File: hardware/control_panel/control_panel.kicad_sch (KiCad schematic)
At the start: 6 parts, among them SW1 RotaryEncoder_Switch_MP, SW2 SW_Push

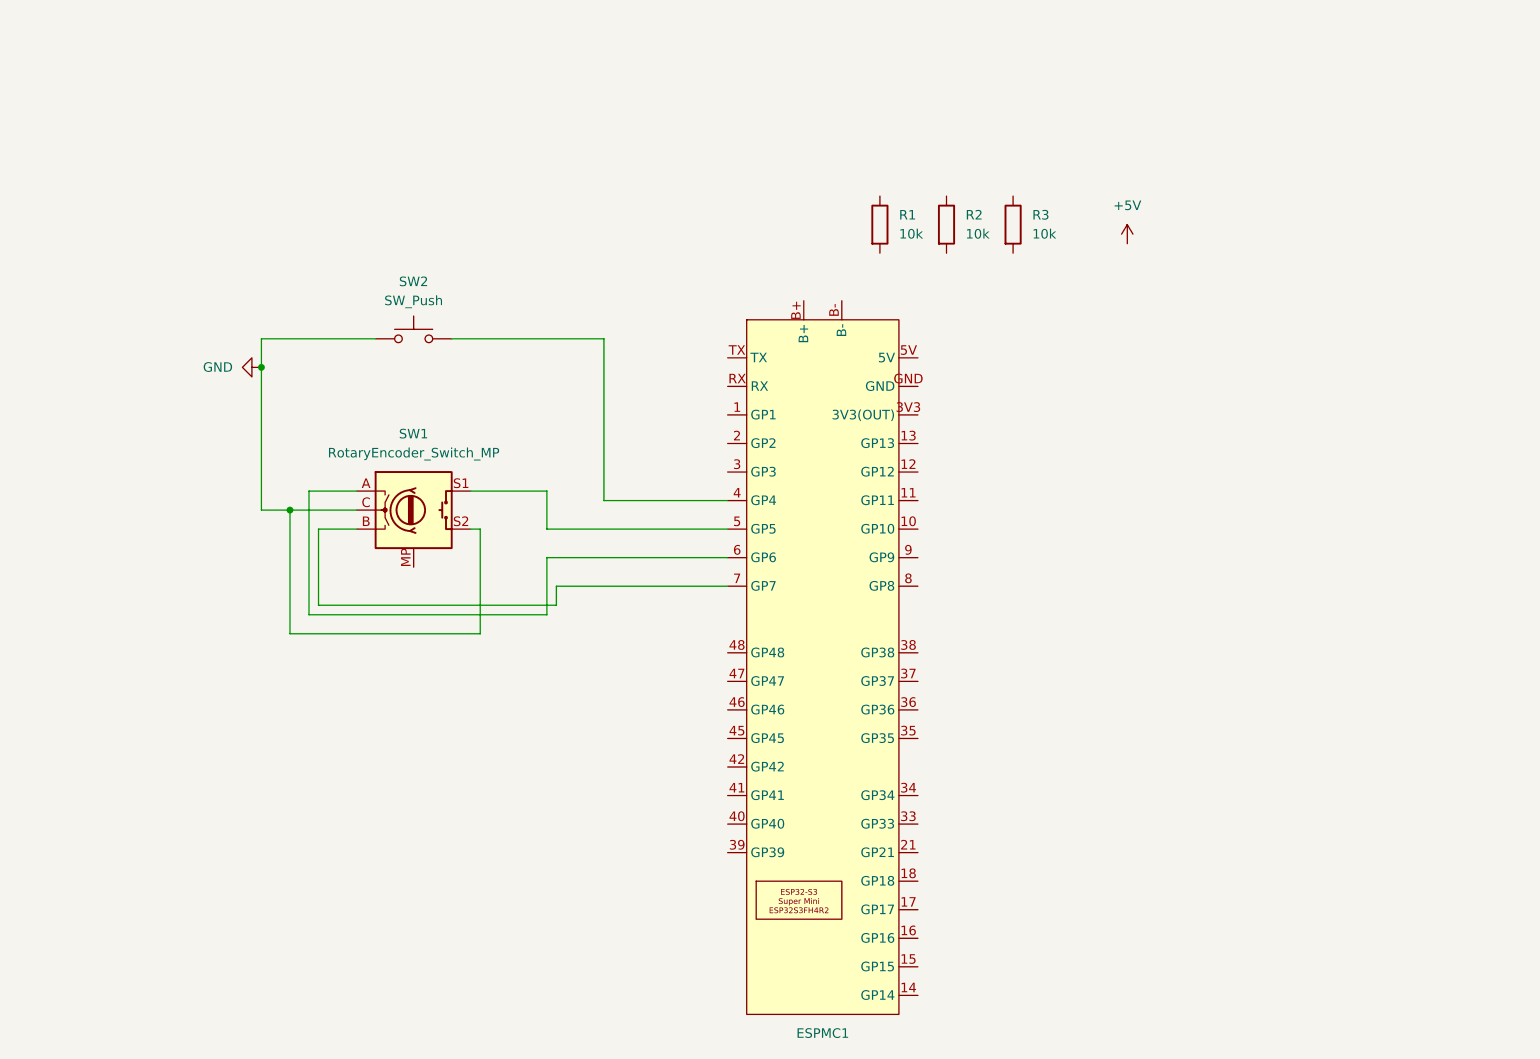
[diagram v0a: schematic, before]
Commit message: KiCad updates and EC11 to TWT
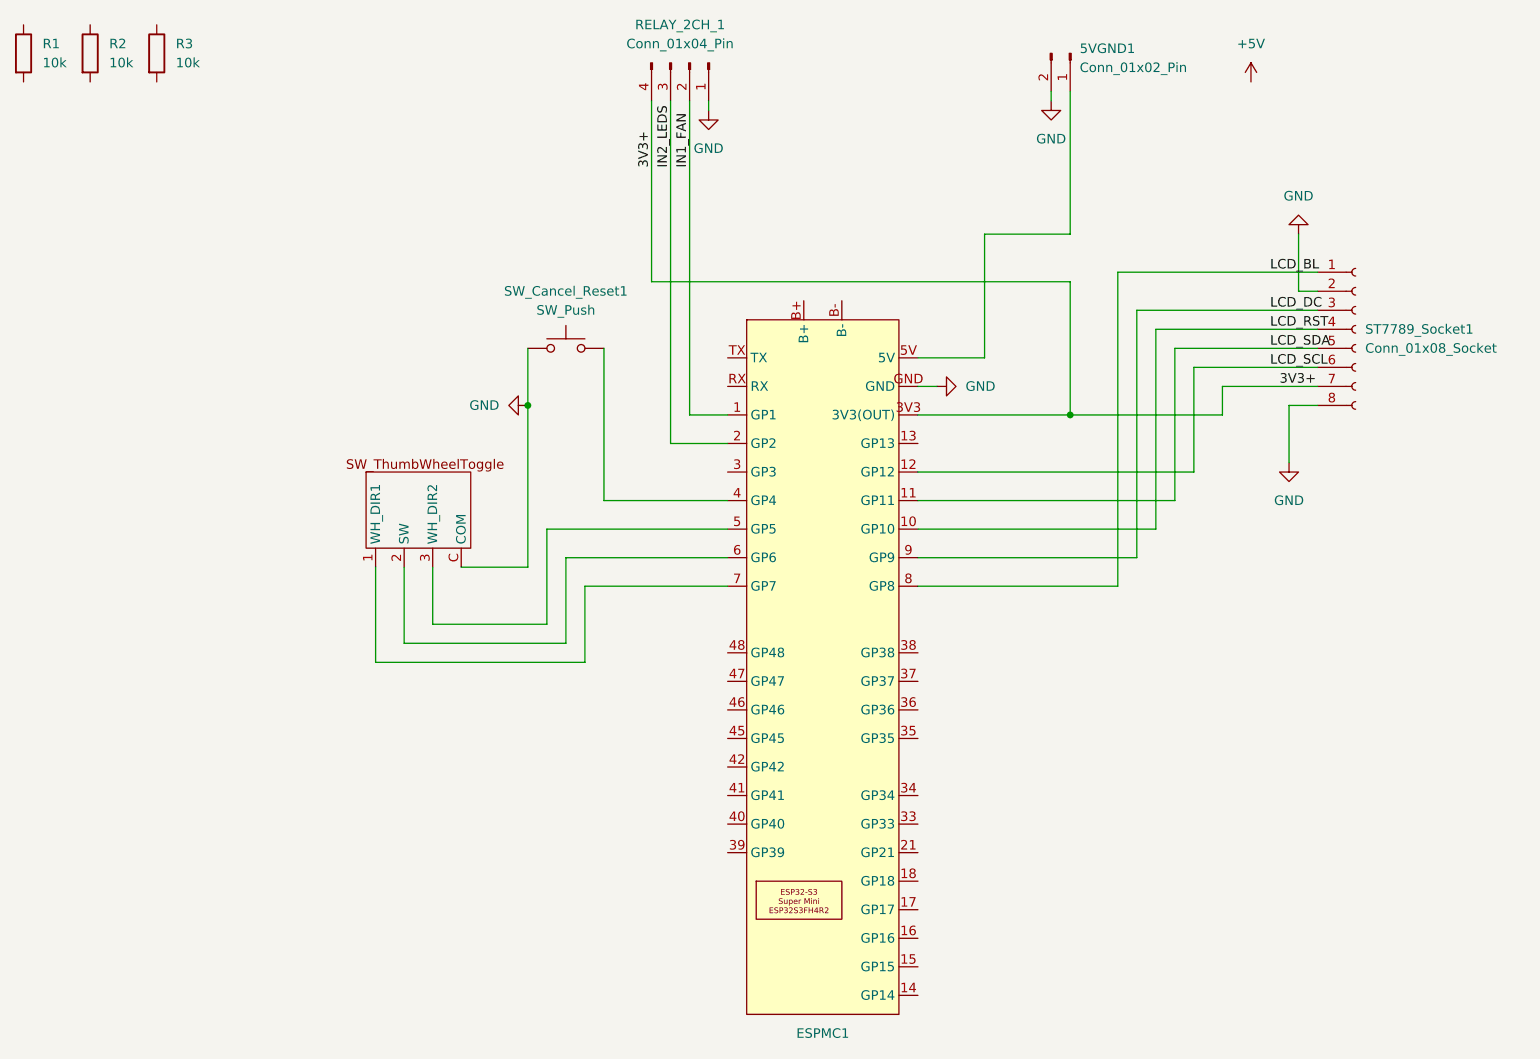
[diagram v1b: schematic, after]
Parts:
- removed SW1: RotaryEncoder_Switch_MP, Rotary_Encoder:RotaryEncoder_Alps_EC11E-Switch_Vertical_H20mm, symbol Device:RotaryEncoder_Switch_MP
- added 5VGND1: Conn_01x02_Pin, Connector_JST:JST_XH_B2B-XH-A_1x02_P2.50mm_Vertical, symbol Connector:Conn_01x02_Pin
- added RELAY_2CH_1: Conn_01x04_Pin, Connector_PinHeader_2.54mm:PinHeader_1x04_P2.54mm_Vertical, symbol Connector:Conn_01x04_Pin
- added ST7789_Socket1: Conn_01x08_Socket, Connector_PinSocket_2.54mm:PinSocket_1x08_P2.54mm_Horizontal, symbol Connector:Conn_01x08_Socket
- added U1: ~, symbol TMB_Library:SW_ThumbWheelToggle
- renumbered SW2 to SW_Cancel_Reset1
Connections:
- net GND: now also ESPMC1.GND, 5VGND1.2 (Pin_2), RELAY_2CH_1.1 (Pin_1), ST7789_Socket1.2 (Pin_2), ST7789_Socket1.8 (Pin_8), U1.C (COM)
- net IN1_FAN: now reaches ESPMC1.1 (GP1)
- net IN1_FAN: now also RELAY_2CH_1.2 (Pin_2)
- net LCD_RST: now reaches ESPMC1.10 (GP10)
- net LCD_RST: now also ST7789_Socket1.4 (Pin_4)
- net LCD_SDA: now reaches ESPMC1.11 (GP11)
- net LCD_SDA: now also ST7789_Socket1.5 (Pin_5)
- net LCD_SCL: now reaches ESPMC1.12 (GP12)
- net LCD_SCL: now also ST7789_Socket1.6 (Pin_6)
- net IN2_LEDS: now reaches ESPMC1.2 (GP2)
- net IN2_LEDS: now also RELAY_2CH_1.3 (Pin_3)
- net 3V3+: now reaches ESPMC1.3V3 (3V3(OUT))
- net 3V3+: now also RELAY_2CH_1.4 (Pin_4), ST7789_Socket1.7 (Pin_7)
- net at ESPMC1.5 (GP5): now also U1.3 (WH_DIR2)
- net at ESPMC1.5V: now also 5VGND1.1 (Pin_1)
- net at ESPMC1.6 (GP6): now also U1.2 (SW)
- net at ESPMC1.7 (GP7): now also U1.1 (WH_DIR1)
- net LCD_BL: now reaches ESPMC1.8 (GP8)
- net LCD_BL: now also ST7789_Socket1.1 (Pin_1)
- net LCD_DC: now reaches ESPMC1.9 (GP9)
- net LCD_DC: now also ST7789_Socket1.3 (Pin_3)
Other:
- moved on the sheet: R1, R2, R3, SW_Cancel_Reset1
